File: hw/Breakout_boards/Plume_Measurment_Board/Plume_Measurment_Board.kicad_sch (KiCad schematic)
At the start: 15 parts, among them J1 Conn_Coaxial, U1 AD7124-8BCPZ-RL

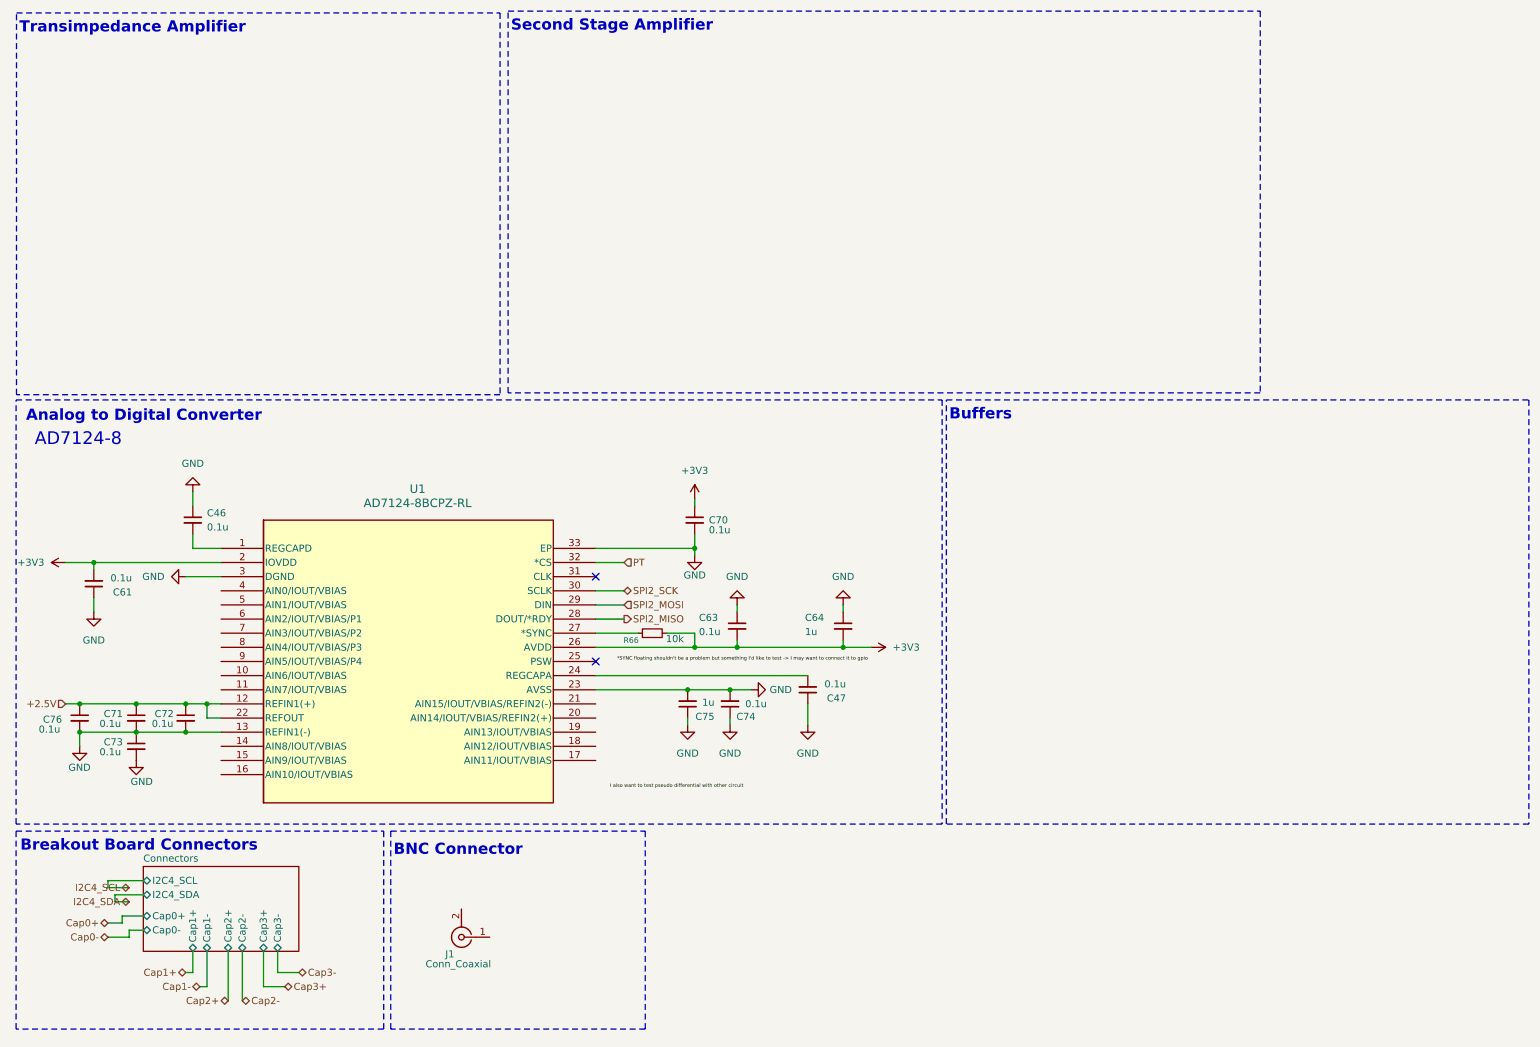
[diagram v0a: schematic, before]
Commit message: Breakout Boards Measurements
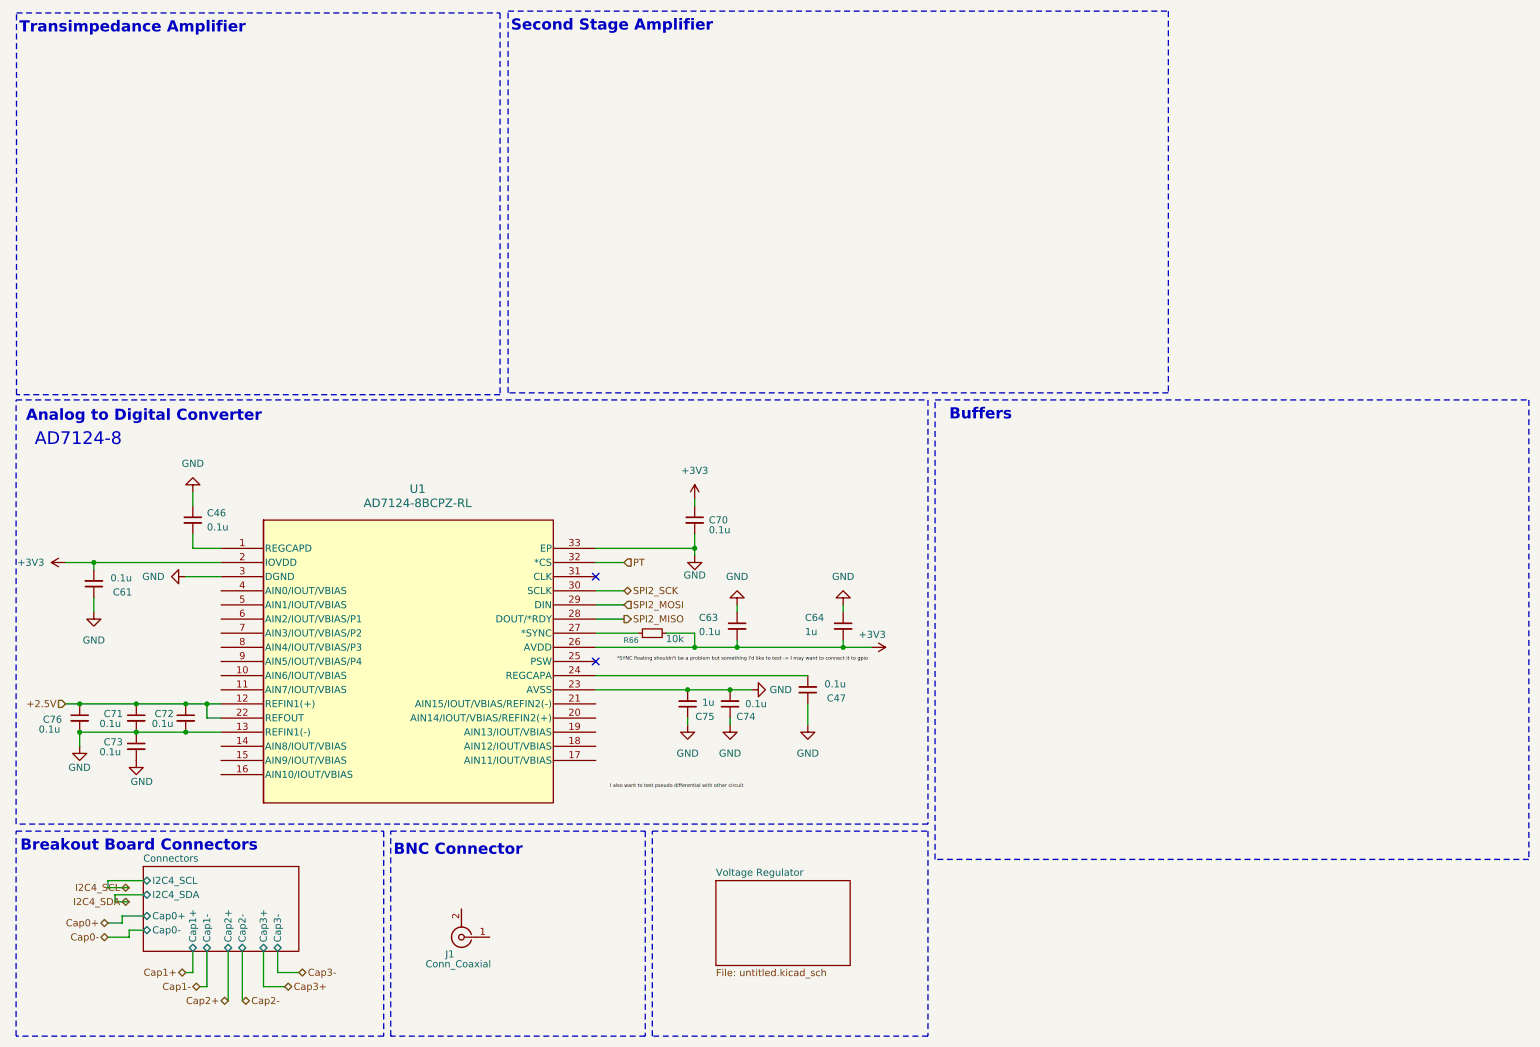
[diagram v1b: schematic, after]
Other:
- added sheet Voltage Regulator (untitled.kicad_sch)
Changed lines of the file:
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@@
 	(rectangle
 		(start 101.092 12.7)
-		(end 236.22 81.28)
+		(end 219.71 81.28)
 		(stroke
 			(width 0)
@@
 	(rectangle
 		(start 12.7 160.02)
-		(end 78.74 195.58)
+		(end 78.74 196.85)
 		(stroke
 			(width 0)
@@
 	)
 	(rectangle
+		(start 127 160.02)
+		(end 176.53 196.85)
+		(stroke
+			(width 0)
+			(type dash)
+		)
+		(fill
+			(type none)
+		)
+	)
+	(rectangle
 		(start 12.7 82.55)
-		(end 179.07 158.75)
+		(end 176.53 158.75)
 		(stroke
 			(width 0)
@@
 	)
 	(rectangle
-		(start 179.832 82.55)
-		(end 284.48 158.75)
+		(start 177.8 82.55)
+		(end 284.48 165.1)
 		(stroke
 			(width 0)
@@
 	(rectangle
 		(start 80.01 160.02)
-		(end 125.73 195.58)
+		(end 125.73 196.85)
 		(stroke
 			(width 0)
@@
 		(in_pos_files yes)
 		(dnp no)
-		(fields_autoplaced yes)
 		(property "Reference" "#PWR0229"
 			(at 162.56 127 0)
@@
 		)
 		(property "Value" "+3V3"
-			(at 170.18 126.9999 90)
+			(at 164.084 124.714 90)
 			(show_name no)
 			(do_not_autoplace no)
@@
 				)
 			)
+		)
+	)
+	(sheet
+		(at 138.43 168.91)
+		(size 24.13 15.24)
+		(exclude_from_sim no)
+		(in_bom yes)
+		(on_board yes)
+		(dnp no)
+		(fields_autoplaced yes)
+		(stroke
+			(width 0.1524)
+			(type solid)
+		)
+		(fill
+			(color 0 0 0 0)
+		)
+		(property "Sheetname" "Voltage Regulator"
+			(at 138.43 168.1984 0)
+			(show_name no)
+			(do_not_autoplace no)
+			(effects
+				(font
+					(size 1.27 1.27)
+				)
+				(justify left bottom)
+			)
+		)
+		(property "Sheetfile" "untitled.kicad_sch"
+			(at 138.43 184.7346 0)
+			(show_name no)
+			(do_not_autoplace no)
+			(effects
+				(font
+					(size 1.27 1.27)
+				)
+				(justify left top)
+			)
+		)
+		(instances
+			(project "Plume_Measurment_Board"
+				(path "/2e1d3673-27b9-4604-80fb-036cec98a912"
+					(page "3")
+				)
+			)
